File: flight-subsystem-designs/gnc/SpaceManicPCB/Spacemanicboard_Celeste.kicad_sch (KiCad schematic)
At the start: 1 part

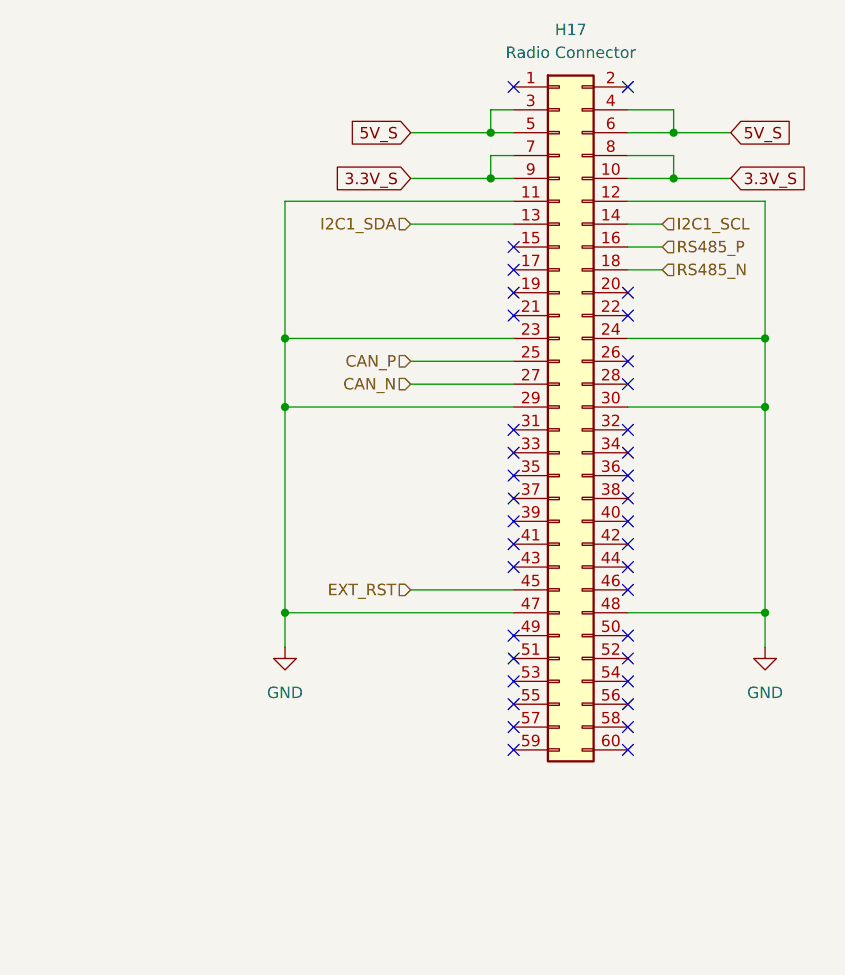
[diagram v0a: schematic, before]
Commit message: Final Changes
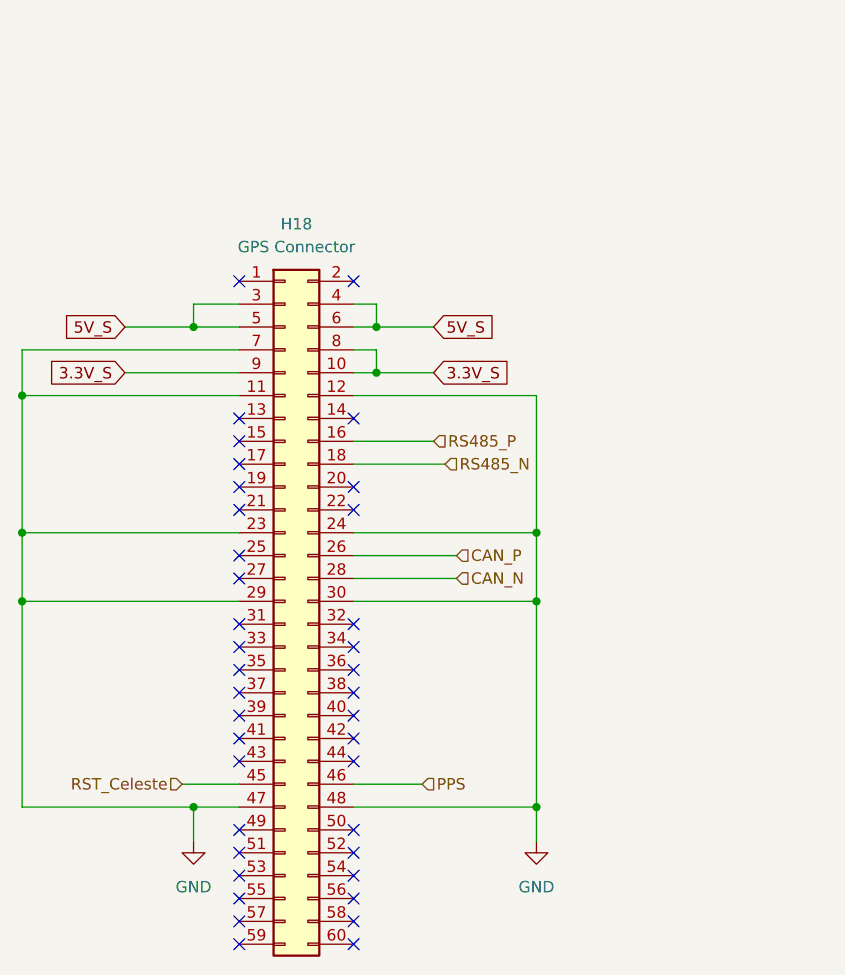
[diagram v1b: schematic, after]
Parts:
- removed H17: Radio Connector, Connector_Molex:CON_MolexSlimStack_54363-0689, symbol Connector_Generic:Conn_02x30_Odd_Even
- added H18: GPS Connector, Connector_Molex:CON_MolexSlimStack_54363-0689, symbol Connector_Generic:Conn_02x30_Odd_Even
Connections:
- net 3.3V_S: now also H18.10 (Pin_10), H18.8 (Pin_8), H18.9 (Pin_9)
- net 5V_S: now also H18.3 (Pin_3), H18.4 (Pin_4), H18.5 (Pin_5), H18.6 (Pin_6)
- net CAN_N: now also H18.28 (Pin_28)
- net CAN_P: now also H18.26 (Pin_26)
- net GND: now also H18.11 (Pin_11), H18.12 (Pin_12), H18.23 (Pin_23), H18.24 (Pin_24), H18.29 (Pin_29), H18.30 (Pin_30), H18.47 (Pin_47), H18.48 (Pin_48), H18.7 (Pin_7)
- net RS485_N: now also H18.18 (Pin_18)
- net RS485_P: now also H18.16 (Pin_16)
- new net PPS: H18.46 (Pin_46)
- new net RST_Celeste: H18.45 (Pin_45)
- no-connect marks 37 -> 38
